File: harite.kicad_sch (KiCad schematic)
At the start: 31 parts, among them U1 RP2040_Zero

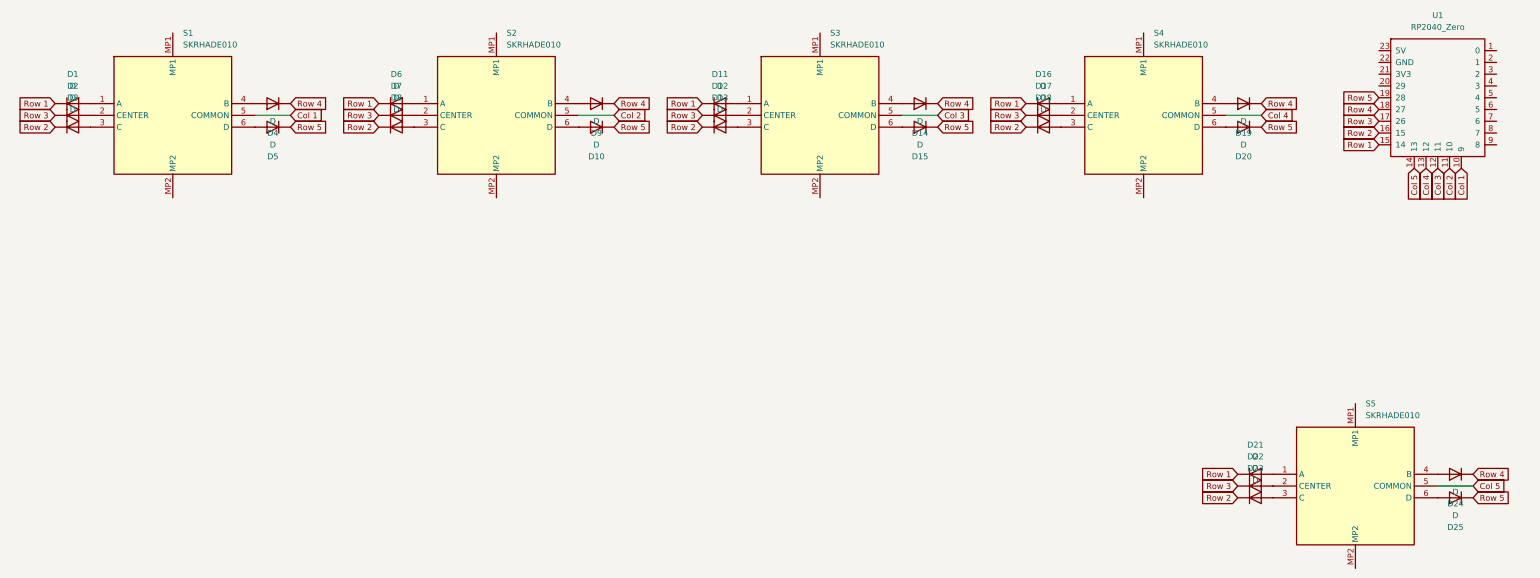
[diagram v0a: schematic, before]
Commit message: Add trrs
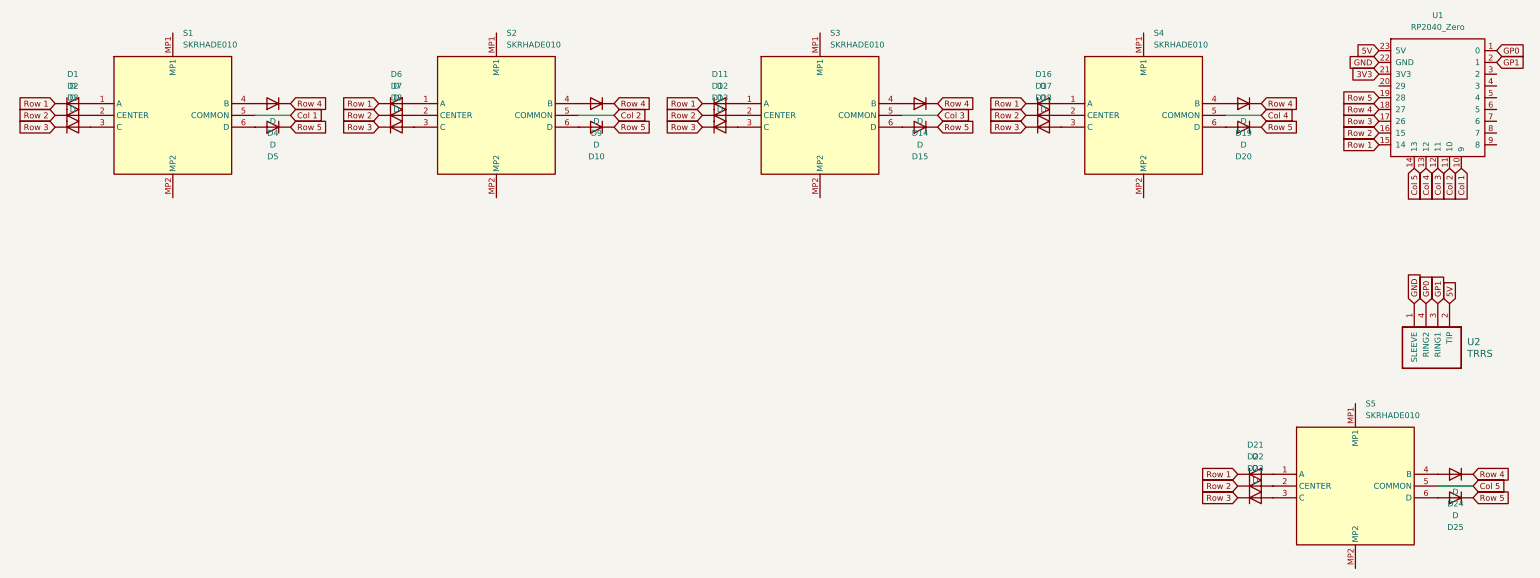
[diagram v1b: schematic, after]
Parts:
- added U2: TRRS, ScottoKeebs_Components:TRRS_PJ-320A, symbol ScottoKeebs:Placeholder_TRRS
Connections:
- net Row 2: now also D12.1 (K), D17.1 (K), D2.1 (K), D22.1 (K), D7.1 (K); no longer D13.1 (K), D18.1 (K), D23.1 (K), D3.1 (K), D8.1 (K)
- net Row 3: now also D13.1 (K), D18.1 (K), D23.1 (K), D3.1 (K), D8.1 (K); no longer D12.1 (K), D17.1 (K), D2.1 (K), D22.1 (K), D7.1 (K)
- net GP0: now reaches U1.1 (0)
- net GP0: now also U2.4 (RING2)
- net GP1: now reaches U1.2 (1)
- net GP1: now also U2.3 (RING1)
- net 3V3: now reaches U1.21 (3V3)
- net GND: now reaches U1.22 (GND)
- net GND: now also U2.1 (SLEEVE)
- net 5V: now reaches U1.23 (5V)
- net 5V: now also U2.2 (TIP)
